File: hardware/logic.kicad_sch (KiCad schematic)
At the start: 19 parts, among them IC1 UCC2946DG4, IC2 SN74LVC1G74DCTR, IC3 SN74LVC1G74DCTR, Q1 BSS123, U1 74157, U2 4011, U3 4081, U4 4071

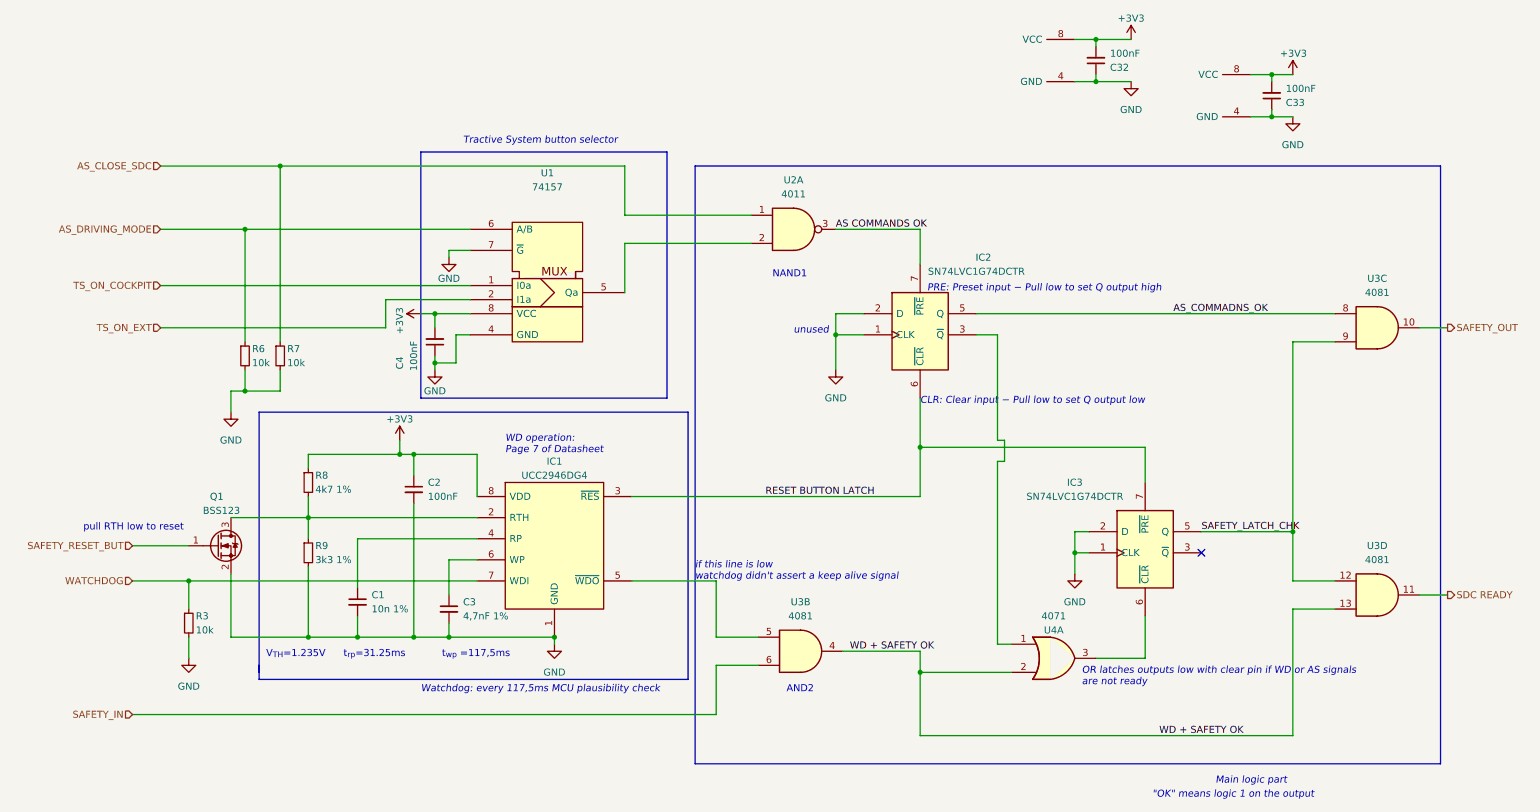
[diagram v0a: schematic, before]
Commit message: L4 port
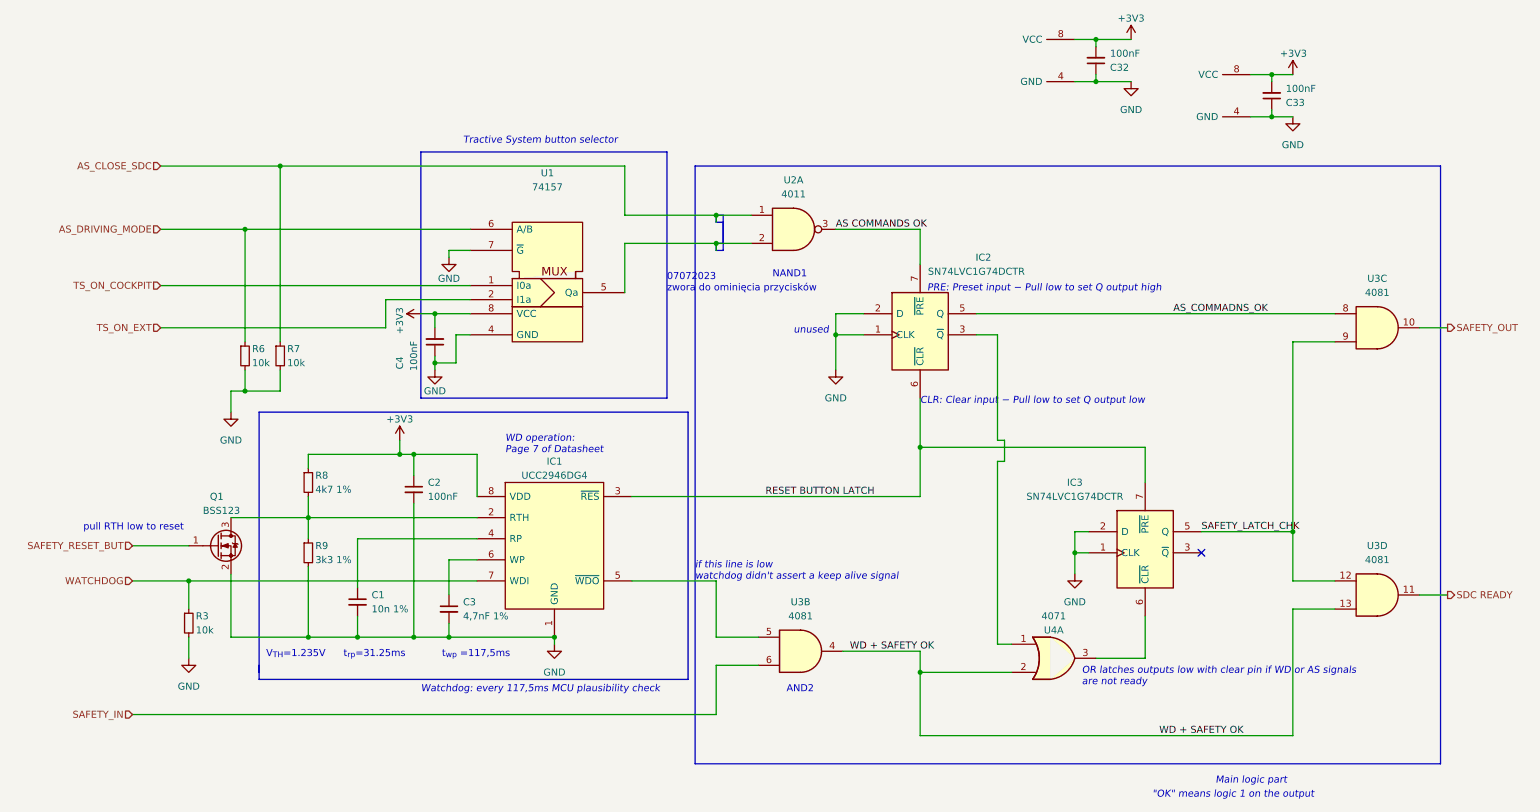
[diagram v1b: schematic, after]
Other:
- note added: "07072023 zwora do ominięcia przycisków"
